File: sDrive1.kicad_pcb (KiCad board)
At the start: 2 copper layers, 50 x 37 mm, 47 parts, among them SW1 SW_Push_Open, U1 DRV8323SRTAT, U2 24LC01

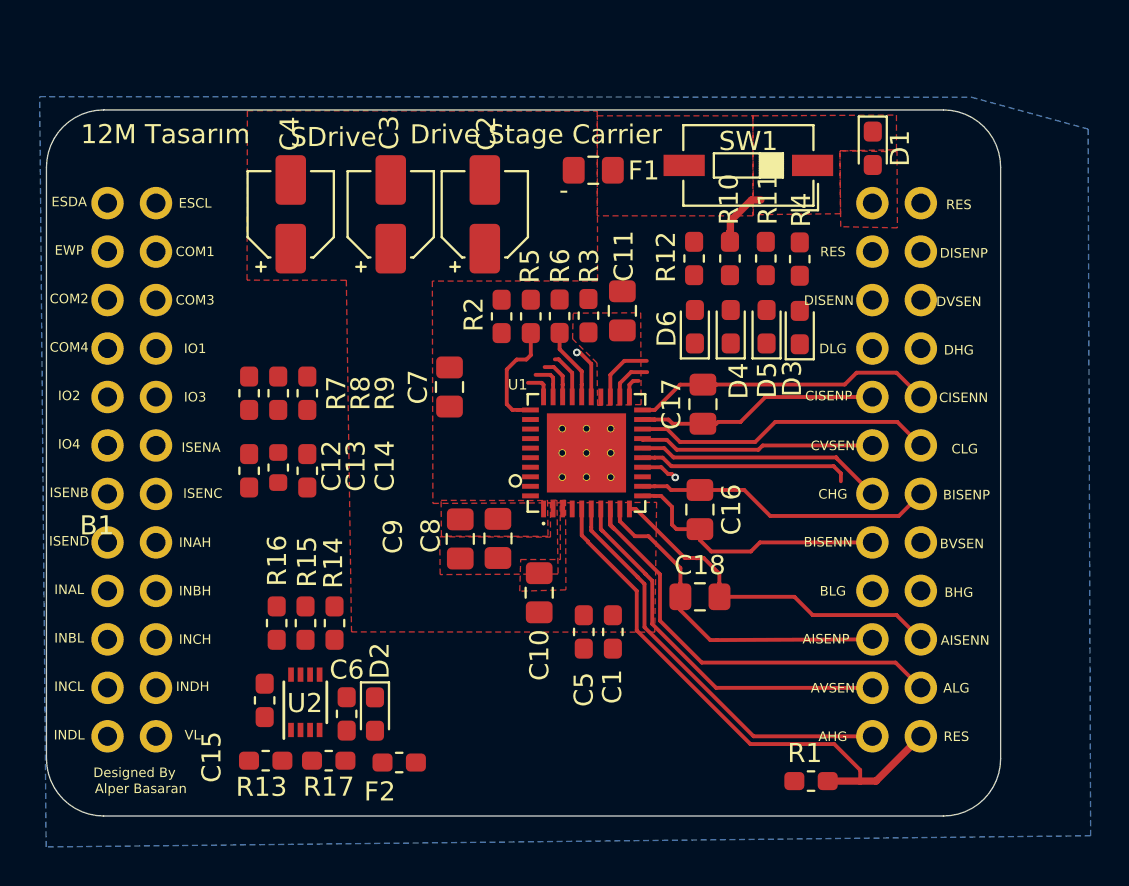
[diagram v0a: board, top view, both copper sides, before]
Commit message: update production files
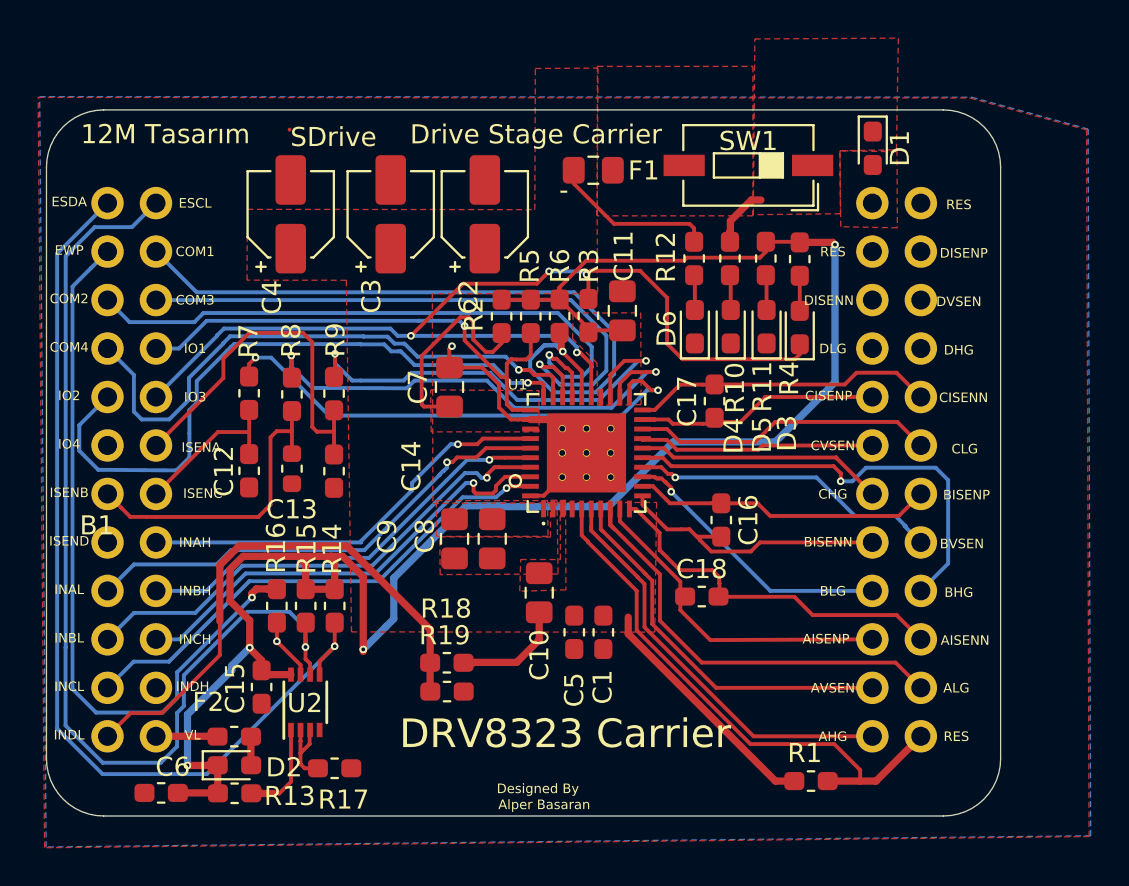
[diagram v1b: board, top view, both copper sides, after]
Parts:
- added R18: R, Resistor_SMD:R_0603_1608Metric_Pad1.05x0.95mm_HandSolder, F.Cu at (20.5, -7.72)
- added R19: R, Resistor_SMD:R_0603_1608Metric_Pad1.05x0.95mm_HandSolder, F.Cu at (20.5, -6.21)
- C16, C17, C18: footprint Capacitor_SMD:C_0805_2012Metric_Pad1.15x1.40mm_HandSolder -> Capacitor_SMD:C_0603_1608Metric_Pad1.05x0.95mm_HandSolder
- moved C6 10.6 mm to (5.55, -0.90), turned to 180 degrees
- moved F2 8.75 mm to (9.38, -3.85), turned to 180 degrees
- moved D2 7.84 mm to (9.39, -2.35), turned to 0 degrees
- moved R13 2.36 mm to (9.40, -0.88)
- moved C14 1.40 mm to (14.6, -17.8)
- moved R7 1.40 mm to (14.6, -21.8)
- moved C16 1.25 mm to (34.9, -15.2)
- moved R16 0.90 mm to (11.6, -10.7)
- moved R14 0.90 mm to (14.6, -10.7)
- moved R15 0.90 mm to (13.1, -10.7)
- moved R8 0.72 mm to (12.4, -21.8)
- moved C13 0.72 mm to (12.4, -17.9)
- moved C15 0.72 mm to (10.8, -6.45)
- moved C17 0.63 mm to (34.5, -21.4)
- moved R17 0.50 mm to (14.6, -2.19)
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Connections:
- B1 pad 23: Net-(B1-Pad23) -> /Drive_Stage/VM_VSEN
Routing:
- net /Drive_Stage/5V: track 0.00 -> 99.8 mm, vias 0 -> 4
- net /Drive_Stage/EEPROM_SCL: track 0.00 -> 53.3 mm, vias 0 -> 1
- net /Drive_Stage/nFAULT: track 2.74 -> 54.9 mm, vias 1 -> 4
- net /Drive_Stage/EEPROM_SDA: track 0.00 -> 50.0 mm, vias 0 -> 1
- net /Drive_Stage/EEPROM_WP: track 0.00 -> 38.5 mm, vias 0 -> 1
- net /Drive_Stage/SDO: track 3.84 -> 42.2 mm, vias 0 -> 1
- net /Drive_Stage/ENABLE: track 1.50 -> 34.6 mm, vias 0 -> 1
- net /Drive_Stage/SDI: track 2.46 -> 33.9 mm, vias 0 -> 1
- net /Drive_Stage/SCLK: track 2.24 -> 33.0 mm, vias 0 -> 1
- net /Drive_Stage/VM_VSEN: track 0.00 -> 28.9 mm
- net /Drive_Stage/NSCS: track 1.99 -> 30.8 mm, vias 0 -> 1
- net /Drive_Stage/VM_Protected: track 0.00 -> 27.4 mm
- net /Drive_Stage/INLC: track 0.00 -> 26.6 mm, vias 0 -> 1
- net /Drive_Stage/INLB: track 0.00 -> 26.2 mm, vias 0 -> 1
- net /Drive_Stage/INLA: track 0.00 -> 25.4 mm, vias 0 -> 1
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- added copper zone on F.Cu, net /Drive_Stage/DVDD
- added copper zone on F.Cu, net GND
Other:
- net class Default: clearance 0.2032 -> 0.1524
- rule trace_clearance: 0.2032 -> 0.1524
- board text added: "DRV8323 Carrier"
